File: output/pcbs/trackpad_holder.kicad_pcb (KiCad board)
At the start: 2 copper layers, 54.1 x 54.1 mm, 4 parts

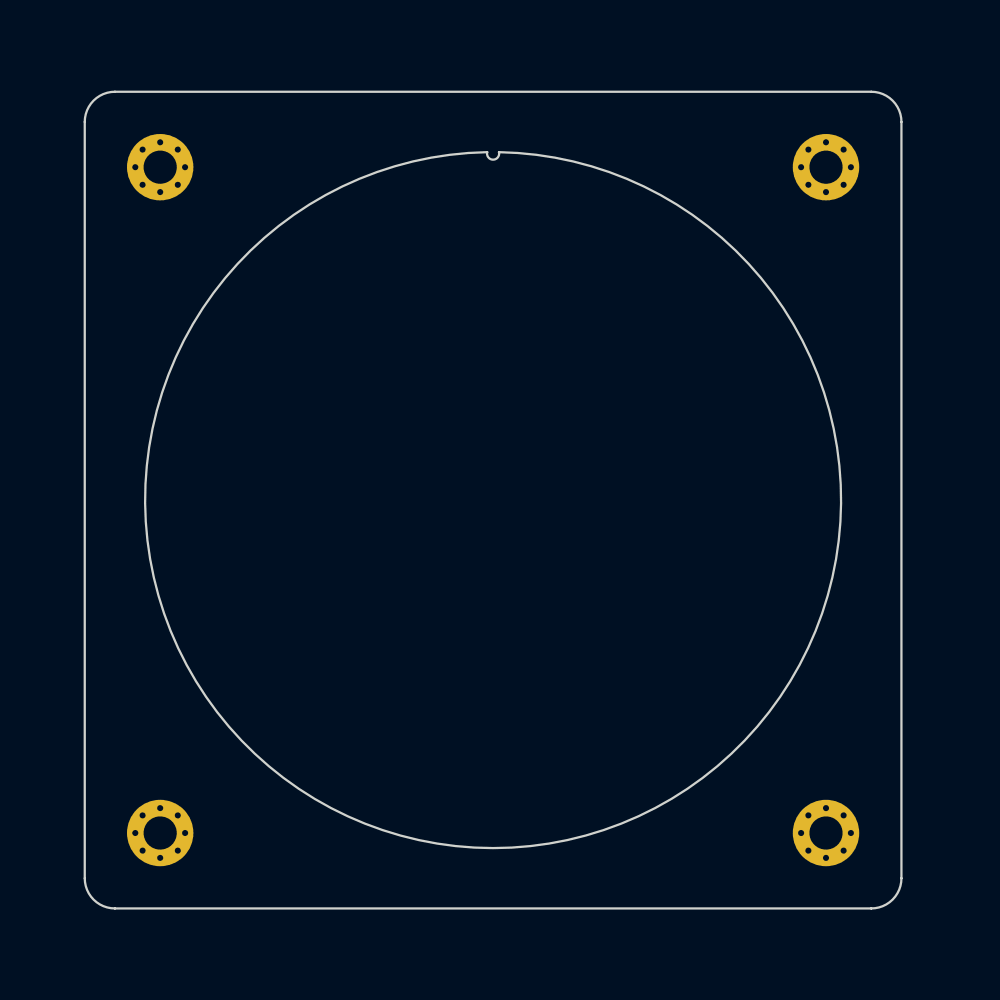
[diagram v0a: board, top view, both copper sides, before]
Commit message: second commit
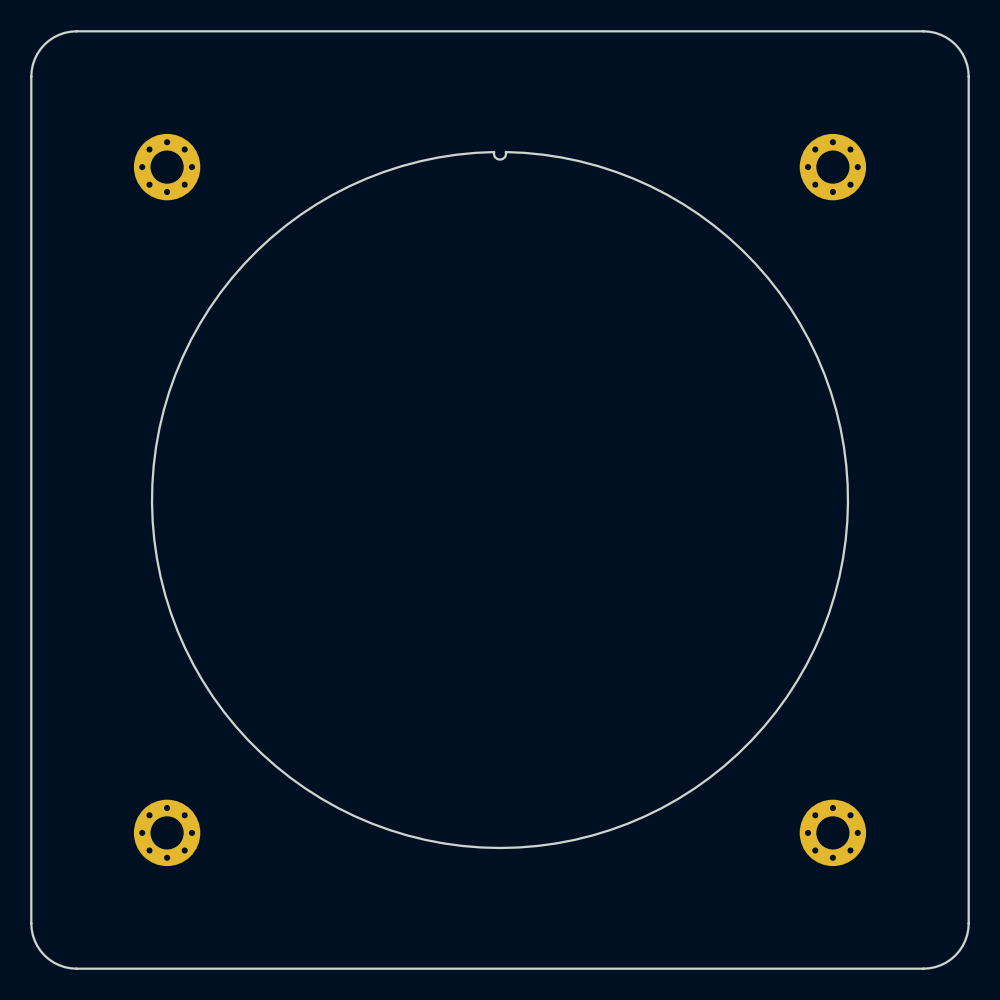
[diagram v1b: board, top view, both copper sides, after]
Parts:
- moved _1 0.46 mm to (227.9, 93.3)
- moved _2 0.46 mm to (183.8, 93.3)
- moved _3 0.46 mm to (227.9, 137.4)
- moved _4 0.46 mm to (183.8, 137.4)
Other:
- board size 54.1 x 54.1 mm -> 62.1 x 62.1 mm
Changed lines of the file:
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@@
   )
     (module "MountingHole_2.2mm_M2_Pad_Via" (version 20210722) (generator pcbnew) (layer "F.Cu")
-      (at 227.4539034 93.2725473 0)
+      (at 227.9113045 93.265776 0)
       (fp_text reference "_1" (at 0 -3.2) (layer "F.SilkS") hide
         (effects (font (size 1 1) (thickness 0.15)))
@@
     )
     (module "MountingHole_2.2mm_M2_Pad_Via" (version 20210722) (generator pcbnew) (layer "F.Cu")
-      (at 183.3239034 93.2725473 0)
+      (at 183.7813045 93.265776 0)
       (fp_text reference "_2" (at 0 -3.2) (layer "F.SilkS") hide
         (effects (font (size 1 1) (thickness 0.15)))
@@
     )
     (module "MountingHole_2.2mm_M2_Pad_Via" (version 20210722) (generator pcbnew) (layer "F.Cu")
-      (at 227.4539034 137.4025473 0)
+      (at 227.9113045 137.395776 0)
       (fp_text reference "_3" (at 0 -3.2) (layer "F.SilkS") hide
         (effects (font (size 1 1) (thickness 0.15)))
@@
     )
     (module "MountingHole_2.2mm_M2_Pad_Via" (version 20210722) (generator pcbnew) (layer "F.Cu")
-      (at 183.3239034 137.4025473 0)
+      (at 183.7813045 137.395776 0)
       (fp_text reference "_4" (at 0 -3.2) (layer "F.SilkS") hide
         (effects (font (size 1 1) (thickness 0.15)))
@@
       (pad "1" thru_hole circle locked (at 0 -1.65) (size 0.7 0.7) (drill 0.4) (layers *.Cu *.Mask))
     )
-  (gr_line (start 180.3239034 142.4025473) (end 230.4539034 142.4025473) (angle 90) (layer Edge.Cuts) (width 0.15))
-(gr_arc (start 230.4539034 140.4025473) (end 230.4539034 142.4025473) (angle -90) (layer Edge.Cuts) (width 0.15))
-(gr_line (start 232.4539034 140.4025473) (end 232.4539034 90.27254730000001) (angle 90) (layer Edge.Cuts) (width 0.15))
-(gr_arc (start 230.4539034 90.27254730000001) (end 232.4539034 90.27254730000001) (angle -90) (layer Edge.Cuts) (width 0.15))
-(gr_line (start 230.4539034 88.27254730000001) (end 180.3239034 88.27254730000001) (angle 90) (layer Edge.Cuts) (width 0.15))
-(gr_arc (start 180.3239034 90.27254730000001) (end 180.3239034 88.27254730000001) (angle -90) (layer Edge.Cuts) (width 0.15))
-(gr_line (start 178.3239034 90.27254730000001) (end 178.3239034 140.4025473) (angle 90) (layer Edge.Cuts) (width 0.15))
-(gr_arc (start 180.3239034 140.4025473) (end 178.3239034 140.4025473) (angle -90) (layer Edge.Cuts) (width 0.15))
-(gr_arc (start 205.3889034 115.3375473) (end 205.0007765 92.2758131) (angle -358.0716164847654) (layer Edge.Cuts) (width 0.15))
-(gr_arc (start 205.3889034 92.3725473) (end 205.0007765 92.2758131) (angle -207.9897971867049) (layer Edge.Cuts) (width 0.15))
+  (gr_line (start 177.7813045 146.395776) (end 233.9113045 146.395776) (angle 90) (layer Edge.Cuts) (width 0.15))
+(gr_arc (start 233.9113045 143.395776) (end 233.9113045 146.395776) (angle -90) (layer Edge.Cuts) (width 0.15))
+(gr_line (start 236.9113045 143.395776) (end 236.9113045 87.26577600000002) (angle 90) (layer Edge.Cuts) (width 0.15))
+(gr_arc (start 233.9113045 87.26577600000002) (end 236.9113045 87.26577600000002) (angle -90) (layer Edge.Cuts) (width 0.15))
+(gr_line (start 233.9113045 84.26577600000002) (end 177.7813045 84.26577600000002) (angle 90) (layer Edge.Cuts) (width 0.15))
+(gr_arc (start 177.7813045 87.26577600000002) (end 177.7813045 84.26577600000002) (angle -90) (layer Edge.Cuts) (width 0.15))
+(gr_line (start 174.7813045 87.26577600000002) (end 174.7813045 143.395776) (angle 90) (layer Edge.Cuts) (width 0.15))
+(gr_arc (start 177.7813045 143.395776) (end 174.7813045 143.395776) (angle -90) (layer Edge.Cuts) (width 0.15))
+(gr_arc (start 205.8463045 115.330776) (end 205.4581776 92.2690418) (angle -358.0716164847654) (layer Edge.Cuts) (width 0.15))
+(gr_arc (start 205.8463045 92.365776) (end 205.4581776 92.2690418) (angle -207.9897971867049) (layer Edge.Cuts) (width 0.15))
 )
